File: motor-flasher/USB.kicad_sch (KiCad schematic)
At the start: 11 parts, among them J4 B2B-PH-K-S-GW, J5 TYPE-C 16PIN 2MD(073), SW2 SS12D07VG4NSGAPA_Powermux

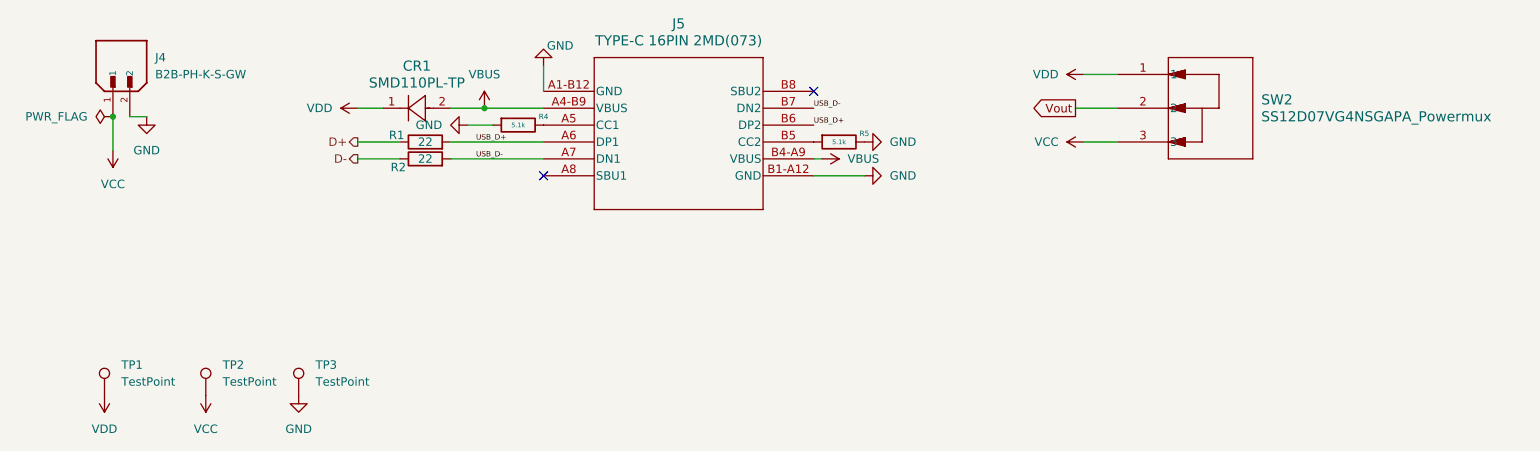
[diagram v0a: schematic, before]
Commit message: Saving current revision
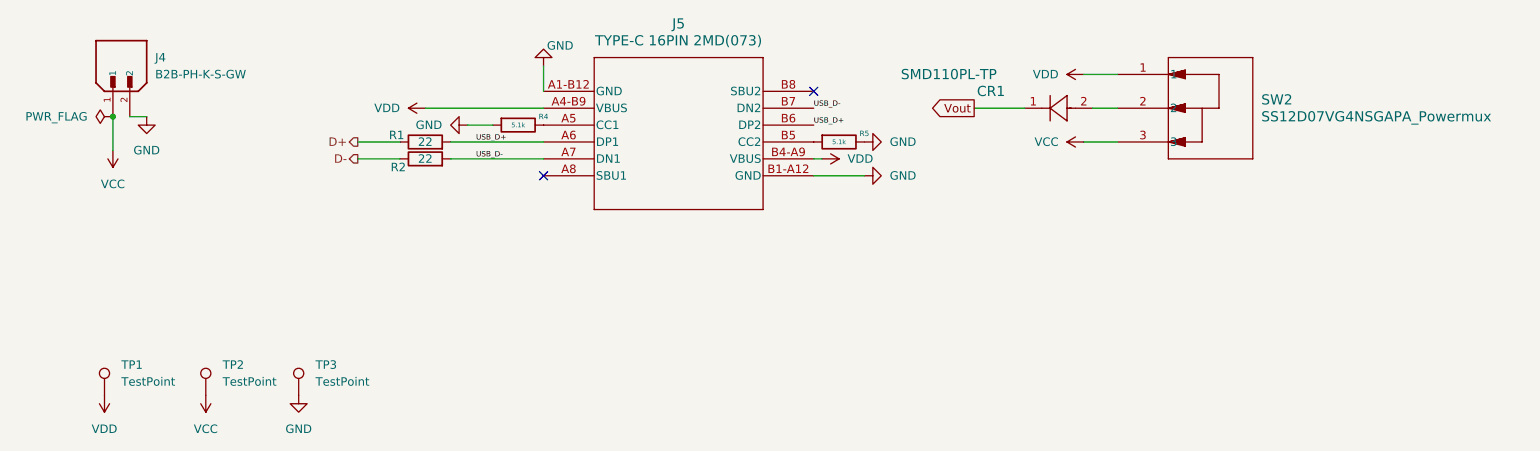
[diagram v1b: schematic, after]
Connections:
- net VDD: now also J5.A4-B9 (VBUS), J5.B4-A9 (VBUS); no longer CR1.1
- net Vout: now also CR1.1; no longer SW2.2
- removed net VBUS: CR1.2, J5.A4-B9 (VBUS), J5.B4-A9 (VBUS)
- new net: CR1.2, SW2.2
